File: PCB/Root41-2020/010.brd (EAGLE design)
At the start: 98 x 70 mm, 127 parts, among them Q1 TO-252-NCH, Q2 TJ8S06M3L, U1 STM32F446RET6, U2 STMICROELECTRONICS_STM32L010F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, U3 STMICROELECTRONICS_STM32L010F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, U4 STMICROELECTRONICS_STM32L010F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, U5 STMICROELECTRONICS_STM32L010F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, X1 B4P-VH, X2 B3B-PH-K-S

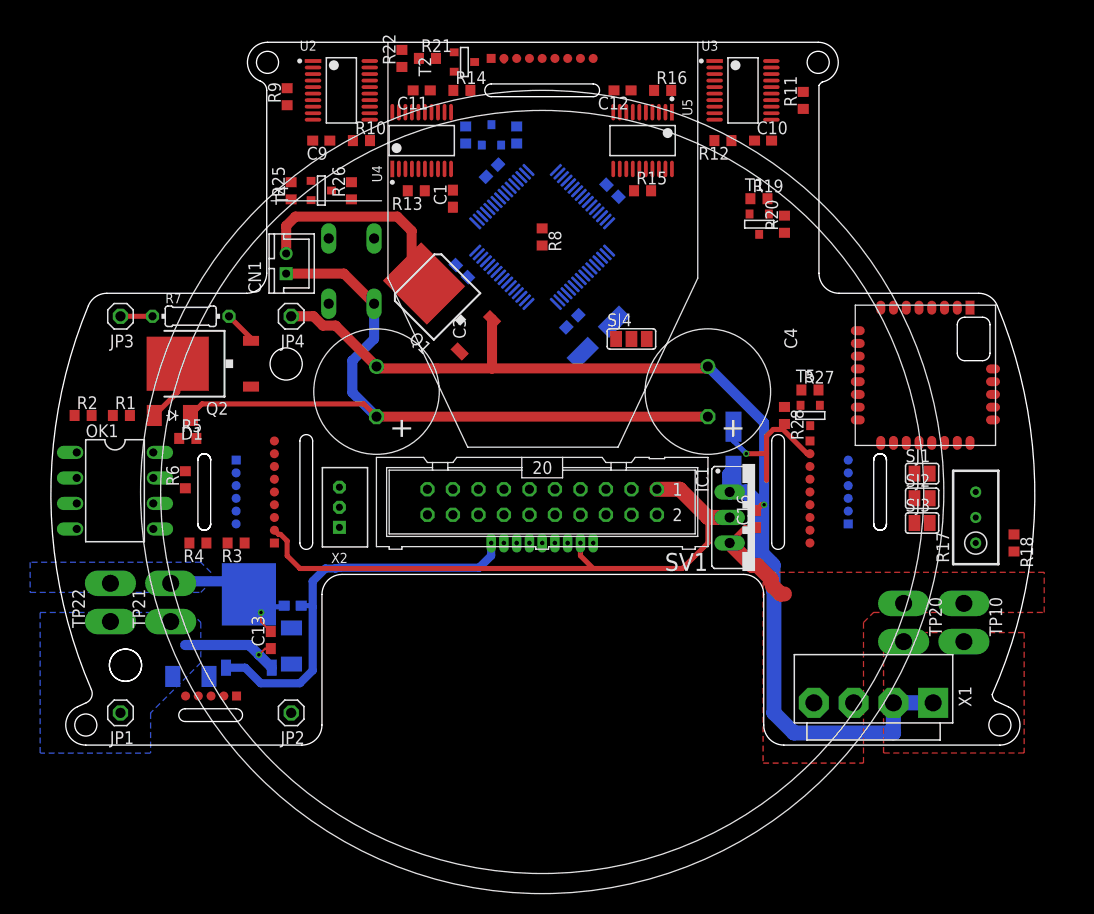
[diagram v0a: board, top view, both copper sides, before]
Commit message: ひとまず配線終わったのだ！疲れたのだ！あとは電源基板とエンコーダ基板だけなのだ！
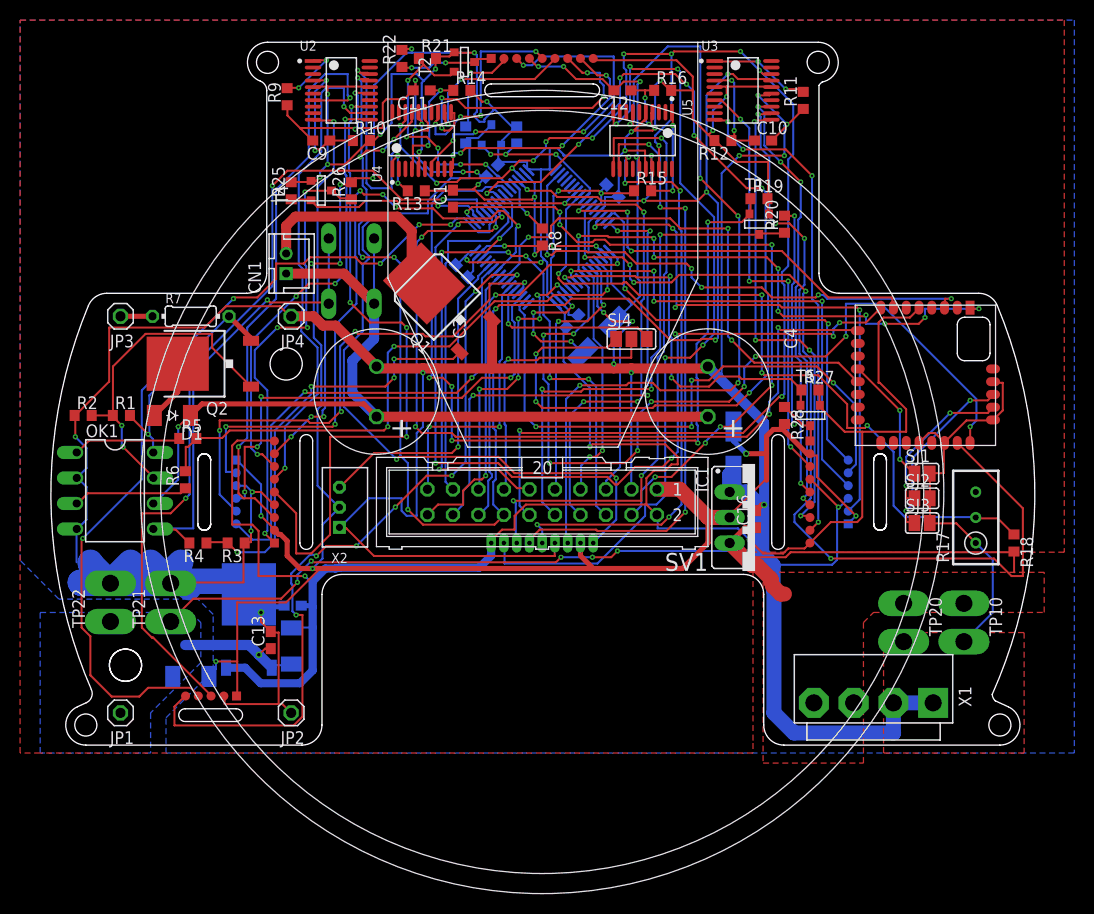
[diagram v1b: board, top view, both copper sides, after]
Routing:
- net GND: track 166.4 -> 606.1 mm, vias 2 -> 31
- net +3V3: track 40.0 -> 367.3 mm, vias 0 -> 20
- net SCL: track 0.00 -> 171.3 mm, vias 0 -> 14
- net SDA: track 0.00 -> 157.1 mm, vias 0 -> 14
- net +5V: track 76.3 -> 226.9 mm, vias 1 -> 13
- net SS-CAM: track 0.00 -> 99.6 mm, vias 0 -> 9
- net RADIO-OUT1: track 0.00 -> 95.3 mm, vias 0 -> 5
- net +12V: track 22.1 -> 114.2 mm, vias 1 -> 7
- net RADIO-RX: track 0.00 -> 91.3 mm, vias 0 -> 7
- net SPK-RX: track 0.00 -> 89.7 mm, vias 0 -> 5
- net NEOPIXEL: track 0.00 -> 87.3 mm, vias 0 -> 5
- net RADIO-OUT2: track 0.00 -> 85.1 mm, vias 0 -> 9
- net SPK-TX: track 0.00 -> 84.9 mm, vias 0 -> 3
- net RADIO-TX: track 0.00 -> 82.6 mm, vias 0 -> 5
- net MUX-B: track 0.00 -> 82.0 mm, vias 0 -> 5
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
